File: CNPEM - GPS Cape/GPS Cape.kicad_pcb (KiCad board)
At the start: 2 copper layers, 11 parts, among them J101 Adafruit_ultimate_GPS_breakout, U101 74LS123

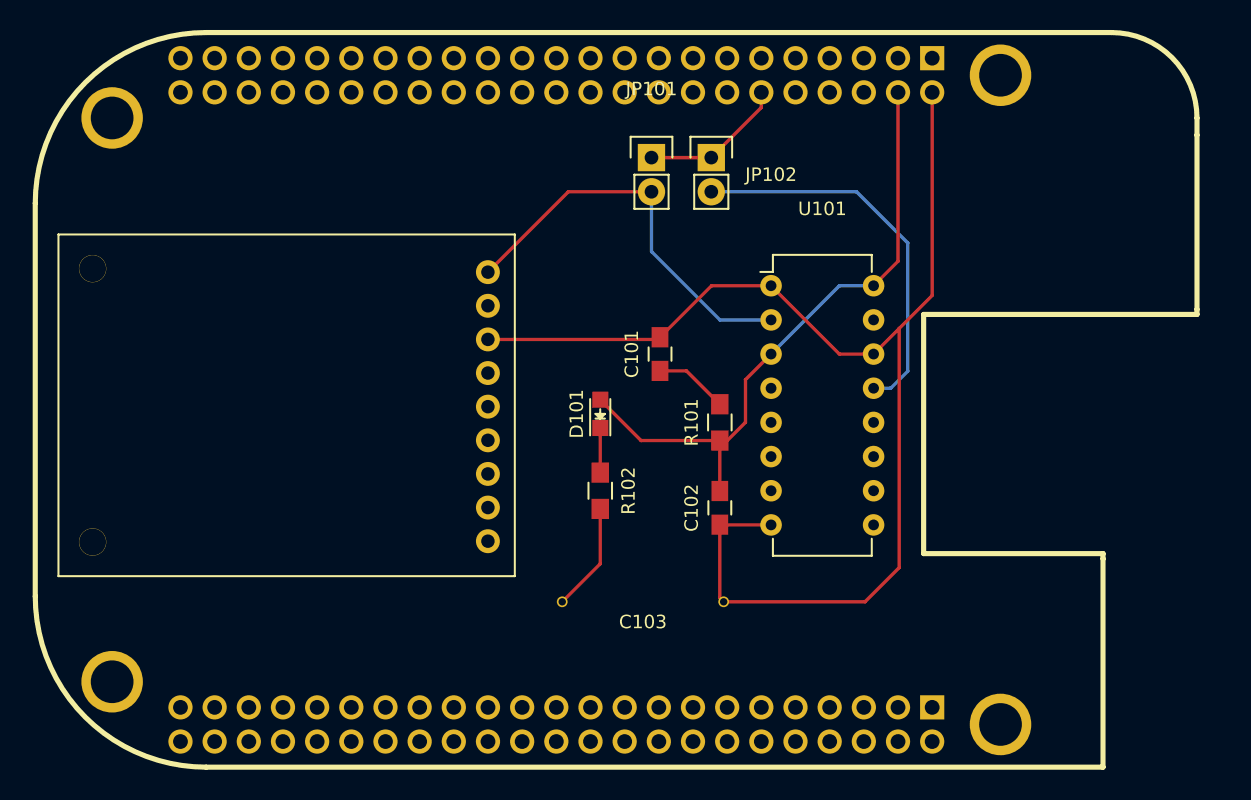
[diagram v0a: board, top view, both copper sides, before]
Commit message: schematics and pcb finished
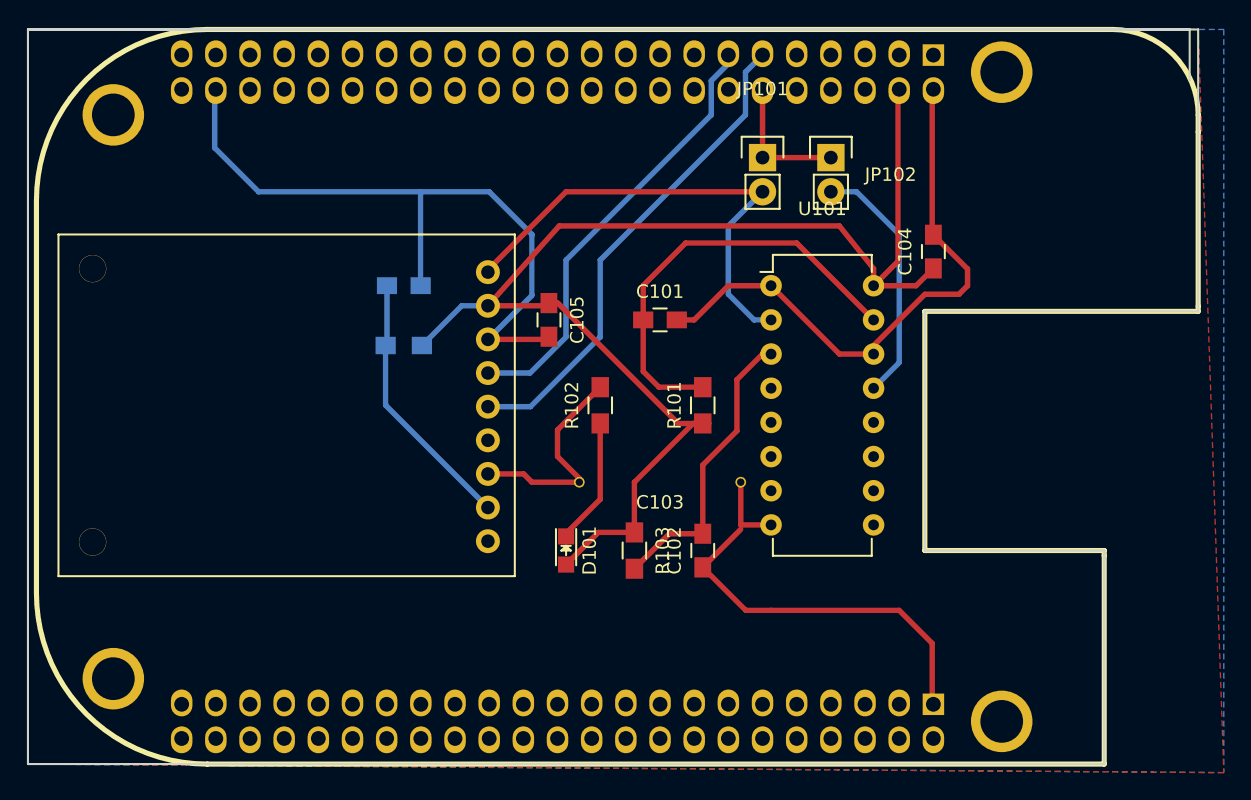
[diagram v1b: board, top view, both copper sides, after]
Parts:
- added C104: 100n, Capacitors_SMD:C_0805_HandSoldering, F.Cu at (172.1, 94.0)
- added C105: 100n, Capacitors_SMD:C_0805_HandSoldering, F.Cu at (143.5, 99.1)
- added C106: 0.1u, Capacitors_SMD:C_0805_HandSoldering, B.Cu at (132.7, 96.5)
- added R103: 10k, Resistors_SMD:R_0805_HandSoldering, F.Cu at (149.9, 116.2)
- added R104: 10k, Resistors_SMD:R_0805_HandSoldering, B.Cu at (132.7, 101.0)
- moved D101 10.5 mm to (144.8, 116.2), turned to 270 degrees
- moved C103 8.98 mm to (151.8, 111.1)
- moved JP102 8.89 mm to (164.5, 87.0)
- moved JP101 8.25 mm to (159.4, 87.0)
- moved R102 6.35 mm to (147.3, 105.4), turned to 90 degrees
- moved C102 3.42 mm to (154.9, 116.2)
- moved C101 2.54 mm to (151.8, 99.1), turned to 0 degrees
- moved R101 1.80 mm to (154.9, 105.4)
- moved Beagle101 0.25 mm to (148.6, 104.8)
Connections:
- Beagle101 pad B1: (no net) -> GND
- Beagle101 pad B10: (no net) -> Net-(Beagle101-PadB10)
- Beagle101 pad B11: (no net) -> Net-(Beagle101-PadB11)
- Beagle101 pad B12: (no net) -> Net-(Beagle101-PadB12)
- Beagle101 pad B13: (no net) -> Net-(Beagle101-PadB13)
- Beagle101 pad B14: (no net) -> Net-(Beagle101-PadB14)
- Beagle101 pad B15: (no net) -> Net-(Beagle101-PadB15)
- Beagle101 pad B16: (no net) -> Net-(Beagle101-PadB16)
- Beagle101 pad B17: (no net) -> Net-(Beagle101-PadB17)
- Beagle101 pad B18: (no net) -> Net-(Beagle101-PadB18)
- Beagle101 pad B19: (no net) -> Net-(Beagle101-PadB19)
- Beagle101 pad B2: (no net) -> Net-(Beagle101-PadB2)
- Beagle101 pad B20: (no net) -> Net-(Beagle101-PadB20)
- Beagle101 pad B21: (no net) -> Net-(Beagle101-PadB21)
- Beagle101 pad B22: (no net) -> Net-(Beagle101-PadB22)
- Beagle101 pad B23: (no net) -> Net-(Beagle101-PadB23)
- Beagle101 pad B24: (no net) -> Net-(Beagle101-PadB24)
- Beagle101 pad B25: (no net) -> Net-(Beagle101-PadB25)
- Beagle101 pad B26: (no net) -> Net-(Beagle101-PadB26)
- Beagle101 pad B27: (no net) -> Net-(Beagle101-PadB27)
- Beagle101 pad B28: (no net) -> Net-(Beagle101-PadB28)
- Beagle101 pad B29: (no net) -> Net-(Beagle101-PadB29)
- Beagle101 pad B3: (no net) -> Net-(Beagle101-PadB3)
- Beagle101 pad B30: (no net) -> Net-(Beagle101-PadB30)
- Beagle101 pad B31: (no net) -> Net-(Beagle101-PadB31)
- Beagle101 pad B32: (no net) -> Net-(Beagle101-PadB32)
- Beagle101 pad B33: (no net) -> Net-(Beagle101-PadB33)
- Beagle101 pad B34: (no net) -> Net-(Beagle101-PadB34)
- Beagle101 pad B35: (no net) -> Net-(Beagle101-PadB35)
- Beagle101 pad B36: (no net) -> Net-(Beagle101-PadB36)
- Beagle101 pad B37: (no net) -> Net-(Beagle101-PadB37)
- Beagle101 pad B38: (no net) -> Net-(Beagle101-PadB38)
- Beagle101 pad B39: (no net) -> Net-(Beagle101-PadB39)
- Beagle101 pad B4: (no net) -> Net-(Beagle101-PadB4)
- Beagle101 pad B40: (no net) -> Net-(Beagle101-PadB40)
- Beagle101 pad B41: (no net) -> Net-(Beagle101-PadB41)
- Beagle101 pad B42: (no net) -> Net-(Beagle101-PadB42)
- Beagle101 pad B43: (no net) -> Net-(Beagle101-PadB43)
- Beagle101 pad B44: (no net) -> Net-(Beagle101-PadB44)
- Beagle101 pad B45: (no net) -> Net-(Beagle101-PadB45)
- Beagle101 pad B46: (no net) -> Net-(Beagle101-PadB46)
- Beagle101 pad B5: (no net) -> Net-(Beagle101-PadB5)
- Beagle101 pad B6: (no net) -> Net-(Beagle101-PadB6)
- Beagle101 pad B7: (no net) -> Net-(Beagle101-PadB7)
- Beagle101 pad B8: (no net) -> Net-(Beagle101-PadB8)
- Beagle101 pad B9: (no net) -> Net-(Beagle101-PadB9)
- Beagle101 pad C4: +3V3 -> VCC
- Beagle101 pad C44: Net-(Beagle101-PadC44) -> GND
- C102 pad 2: +3V3 -> Net-(C102-Pad2)
- D101 pad 2: +3V3 -> VCC
- J101 pad 2: +3V3 -> Net-(C106-Pad2)
- J101 pad 8: +3V3 -> VCC
- R101 pad 1: +3V3 -> VCC
- U101 pad 16: +3V3 -> VCC
- U101 pad 3: +3V3 -> Net-(C102-Pad2)
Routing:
- net VCC: track 0.00 -> 97.4 mm
- net +3V3: track 47.1 -> 0.00 mm
- net /TX_GPS: track 0.00 -> 36.4 mm
- net GND: track 95.2 -> 128.3 mm
- net /RX_GPS: track 0.00 -> 32.9 mm
- net Net-(C101-Pad1): track 5.47 -> 32.1 mm
- net Net-(C102-Pad2): track 0.00 -> 22.0 mm
- net Net-(C106-Pad2): track 0.00 -> 19.7 mm
- net /PPS_ENL: track 28.8 -> 18.6 mm
- net Net-(C103-Pad1): track 8.08 -> 16.1 mm
- net Net-(D101-Pad1): track 3.32 -> 9.45 mm
- net /PPS: track 30.2 -> 35.6 mm
- net Net-(Beagle101-PadC12): track 10.8 -> 10.2 mm
- added copper zone on B.Cu, net GND
- added copper zone on F.Cu, net GND
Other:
- board outline added: 87 x 54.6 mm
